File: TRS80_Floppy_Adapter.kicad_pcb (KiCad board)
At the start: 2 copper layers, 40.6 x 76.2 mm, 3 parts

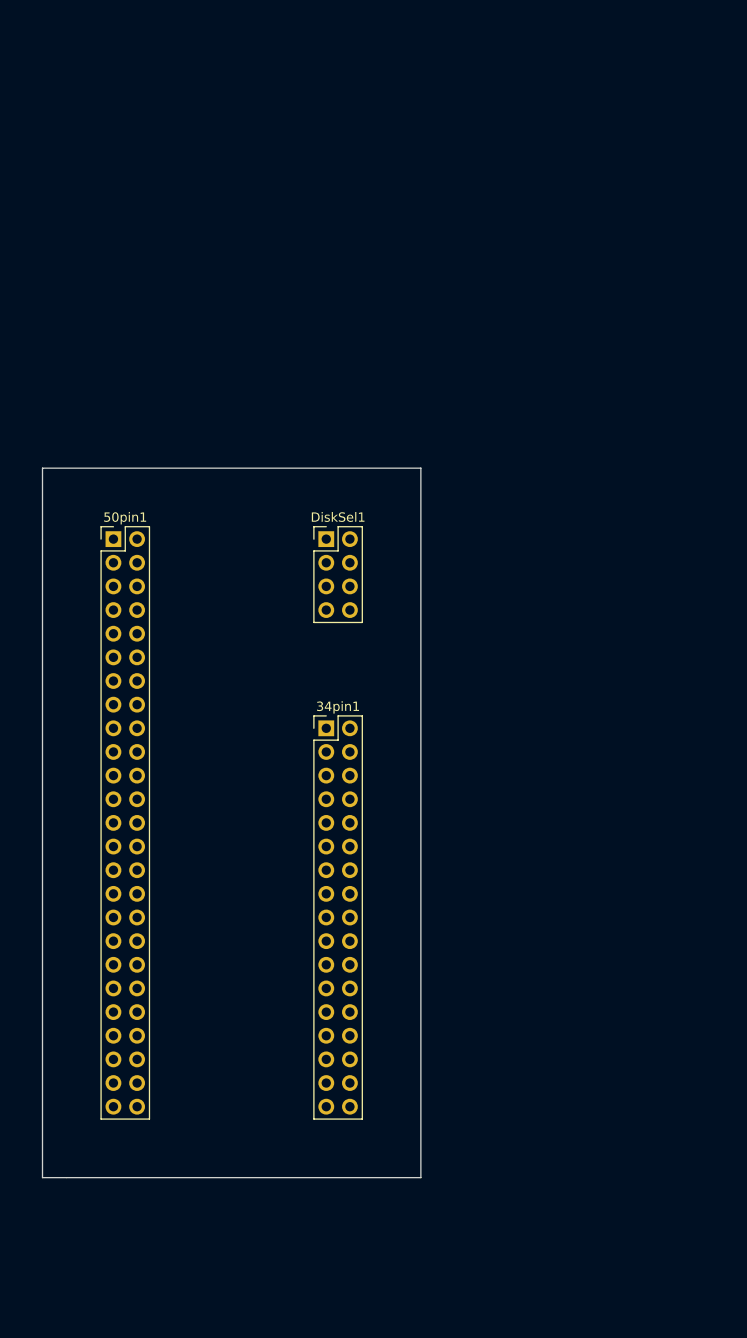
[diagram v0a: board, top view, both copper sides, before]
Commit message: Add files via upload
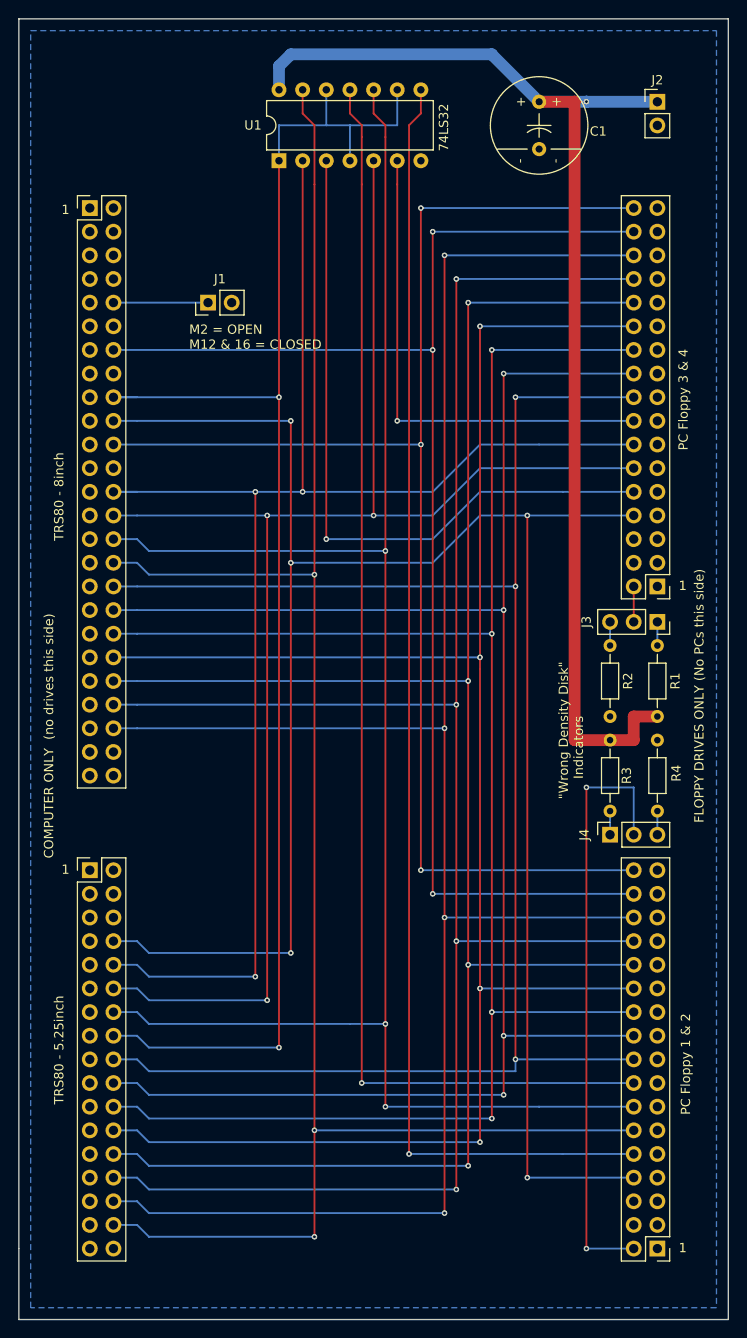
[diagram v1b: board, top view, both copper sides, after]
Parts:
- removed 34pin1: Conn_02x17_Odd_Even, Connector_PinHeader_2.54mm:PinHeader_2x17_P2.54mm_Vertical
- removed 50pin1: Conn_02x25_Odd_Even, Connector_PinHeader_2.54mm:PinHeader_2x25_P2.54mm_Vertical
- removed DiskSel1: Conn_02x04_Odd_Even, Connector_PinHeader_2.54mm:PinHeader_2x04_P2.54mm_Vertical
- added C1: Capacitor, GenericComponents:Capcitor Radial .200, F.Cu at (137.2, 24.1)
- added J1: Conn_02x01, Connector_PinHeader_2.54mm:PinHeader_1x02_P2.54mm_Vertical, F.Cu at (109.2, 50.8)
- added J2: Conn_02x01, Connector_PinHeader_2.54mm:PinHeader_1x02_P2.54mm_Vertical, F.Cu at (157.5, 29.2)
- added J3: Conn_01x03_Socket, Connector_PinSocket_2.54mm:PinSocket_1x03_P2.54mm_Vertical, F.Cu at (157.5, 85.1)
- added J4: Conn_01x03_Socket, Connector_PinSocket_2.54mm:PinSocket_1x03_P2.54mm_Vertical, F.Cu at (152.4, 108.0)
- added PC Floppy 1 & 2: Conn_02x17_Odd_Even, Connector_PinHeader_2.54mm:PinHeader_2x17_P2.54mm_Vertical, F.Cu at (157.5, 152.4)
- added PC Floppy 3 & 4: Conn_02x17_Odd_Even, Connector_PinHeader_2.54mm:PinHeader_2x17_P2.54mm_Vertical, F.Cu at (157.5, 81.3)
- added R1: Resistor, Resistor_THT:R_Axial_DIN0204_L3.6mm_D1.6mm_P7.62mm_Horizontal, F.Cu at (157.5, 87.6)
- added R2: Resistor, Resistor_THT:R_Axial_DIN0204_L3.6mm_D1.6mm_P7.62mm_Horizontal, F.Cu at (152.4, 87.6)
- added R3: Resistor, Resistor_THT:R_Axial_DIN0204_L3.6mm_D1.6mm_P7.62mm_Horizontal, F.Cu at (152.4, 105.4)
- added R4: Resistor, Resistor_THT:R_Axial_DIN0204_L3.6mm_D1.6mm_P7.62mm_Horizontal, F.Cu at (157.5, 105.4)
- added TRS80 - 5.25inch: Conn_02x17_Odd_Even, Connector_PinHeader_2.54mm:PinHeader_2x17_P2.54mm_Vertical, F.Cu at (96.5, 111.8)
- added TRS80 - 8inch: Conn_02x25_Odd_Even, Connector_PinHeader_2.54mm:PinHeader_2x25_P2.54mm_Vertical, F.Cu at (96.5, 40.6)
- added U1: 74LS32, GenericComponents:DIP-14pin, F.Cu at (116.8, 35.6)
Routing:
- net Net-(PC_5inch1-Pin_8): track 0.00 -> 217.3 mm, vias 0 -> 5
- net Net-(PC_5inch1-Pin_30): track 0.00 -> 215.2 mm, vias 0 -> 4
- net Net-(PC_5inch1-Pin_28): track 0.00 -> 210.1 mm, vias 0 -> 4
- net Net-(PC_5inch1-Pin_26): track 0.00 -> 205.0 mm, vias 0 -> 4
- net Net-(PC_5inch1-Pin_12): track 0.00 -> 202.2 mm, vias 0 -> 3
- net Net-(PC_5inch1-Pin_24): track 0.00 -> 199.9 mm, vias 0 -> 4
- net Net-(PC_5inch1-Pin_14): track 0.00 -> 195.9 mm, vias 0 -> 3
- net Net-(PC_5inch1-Pin_22): track 0.00 -> 194.8 mm, vias 0 -> 4
- net Net-(PC_5inch1-Pin_20): track 0.00 -> 189.8 mm, vias 0 -> 4
- net Net-(PC_5inch1-Pin_18): track 0.00 -> 184.7 mm, vias 0 -> 3
- net Net-(PC_5inch2-Pin_12): track 0.00 -> 165.2 mm, vias 0 -> 3
- net Net-(PC_5inch2-Pin_14): track 0.00 -> 163.9 mm, vias 0 -> 3
- net Net-(TRS80-5inch1-Pin_16): track 0.00 -> 161.8 mm, vias 0 -> 2
- net Net-(PC_5inch1-Pin_34): track 0.00 -> 149.9 mm, vias 0 -> 3
- net Net-(PC_5inch1-Pin_32): track 0.00 -> 148.6 mm, vias 0 -> 3
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- added copper zone on B.Cu, net GND
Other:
- board size 40.6 x 76.2 mm -> 76.2 x 139.7 mm
- board text added: "1"
- board text added: "74LS32"
- board text added: "COMPUTER ONLY (no drives this side)"
- board text added: "FLOPPY DRIVES ONLY (No PCs this side)"
- board text added: "M2 = OPEN M12 & 16 = CLOSED"
- board text added: "{dblquote}Wrong Density Disk{dblquote} Indicators"
